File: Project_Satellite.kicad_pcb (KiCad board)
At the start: 4 copper layers, 40.2 x 65.5 mm, 83 parts, among them J1 Conn_01x02_Socket, J10 Conn_01x01_Socket, J11 Conn_01x01_Socket, J12 Conn_01x01_Socket, J13 Conn_01x01_Socket, J14 Conn_01x01_Socket, J15 Conn_01x01_Socket, J16 Conn_01x01_Socket, J17 Conn_01x01_Socket, J18 Conn_01x01_Socket, J19 Conn_01x01_Socket, J2 Conn_01x01_Socket, J20 Conn_01x01_Socket, J21 Conn_01x01_Socket, J22 Conn_01x01_Socket, J23 Conn_01x01_Socket, J24 Conn_01x01_Socket, J25 Conn_01x03_Socket, J26 Conn_01x03_Socket, J27 Conn_01x03_Socket, J28 Conn_01x03_Socket, J3 Conn_01x01_Socket, J4 Conn_01x01_Socket, J5 Conn_01x02_Socket, J6 Conn_01x02_Socket, J7 Conn_01x01_Socket, J8 Conn_01x02_Socket, J9 Conn_01x02_Socket, U3 TPS62933, U4 RASPBERRY_PI_ZERO_2_W, U5 TLV320AIC3254IRHBR, U6 MEMSMic, U7 MEMSMic, U8 TPA3118D2DAPR

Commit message: Final V1 commit
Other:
- copper layers 4 -> 2
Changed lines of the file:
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@@
 	(layers
 		(0 "F.Cu" signal)
-		(4 "In1.Cu" power "PWR.Cu")
-		(6 "In2.Cu" power "GND.Cu")
 		(2 "B.Cu" signal)
 		(9 "F.Adhes" user "F.Adhesive")
@@
 			)
 			(layer "dielectric 1"
-				(type "prepreg")
-				(thickness 0.1)
-				(material "FR4")
-				(epsilon_r 4.5)
-				(loss_tangent 0.02)
-			)
-			(layer "In1.Cu"
-				(type "copper")
-				(thickness 0.035)
-			)
-			(layer "dielectric 2"
 				(type "core")
-				(thickness 1.24)
-				(material "FR4")
-				(epsilon_r 4.5)
-				(loss_tangent 0.02)
-			)
-			(layer "In2.Cu"
-				(type "copper")
-				(thickness 0.035)
-			)
-			(layer "dielectric 3"
-				(type "prepreg")
-				(thickness 0.1)
+				(thickness 1.51)
 				(material "FR4")
 				(epsilon_r 4.5)
@@
 			(plot_on_all_layers_selection 0x00000000_00000000_00000000_00000000)
 			(disableapertmacros no)
-			(usegerberextensions no)
+			(usegerberextensions yes)
 			(usegerberattributes yes)
 			(usegerberadvancedattributes yes)
@@
 			(outputformat 1)
 			(mirror no)
-			(drillshape 1)
+			(drillshape 0)
 			(scaleselection 1)
-			(outputdirectory "")
+			(outputdirectory "V1_Fabrication/")
 		)
 	)

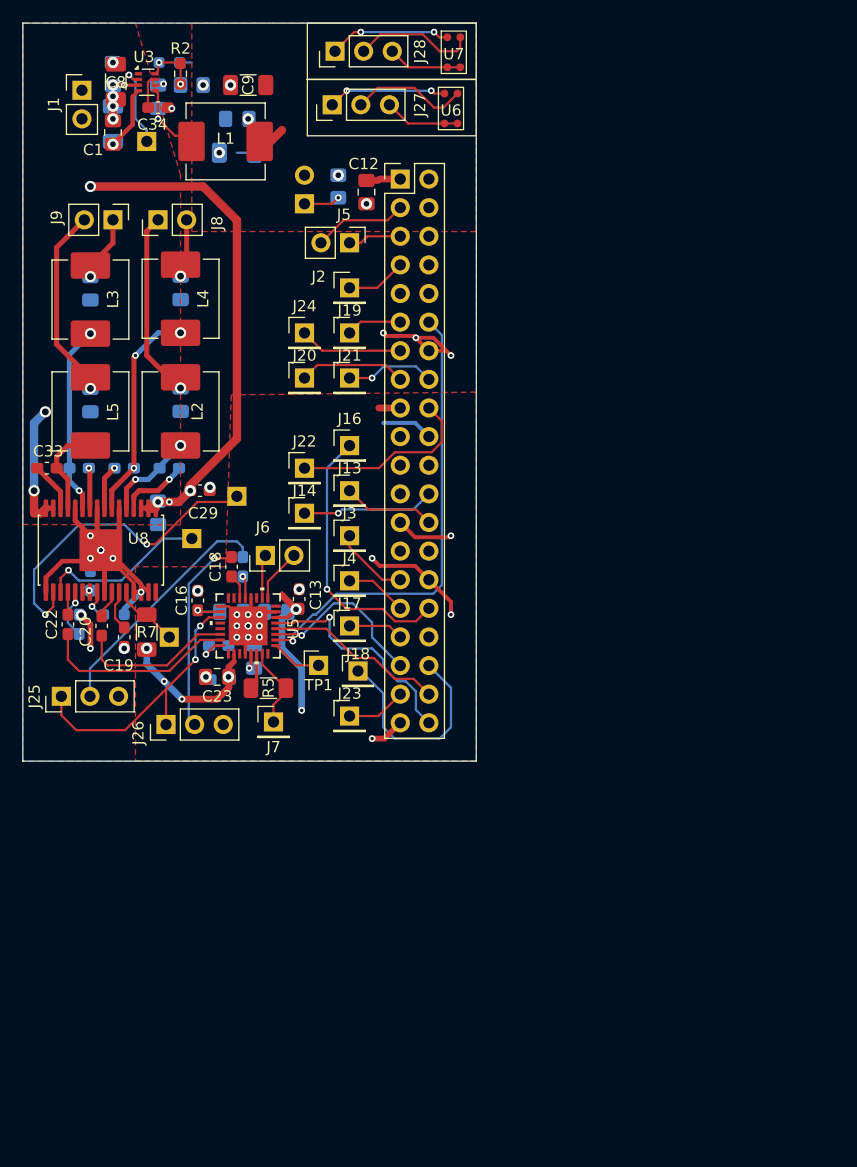
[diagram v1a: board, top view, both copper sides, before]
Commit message: TPA3118 changes
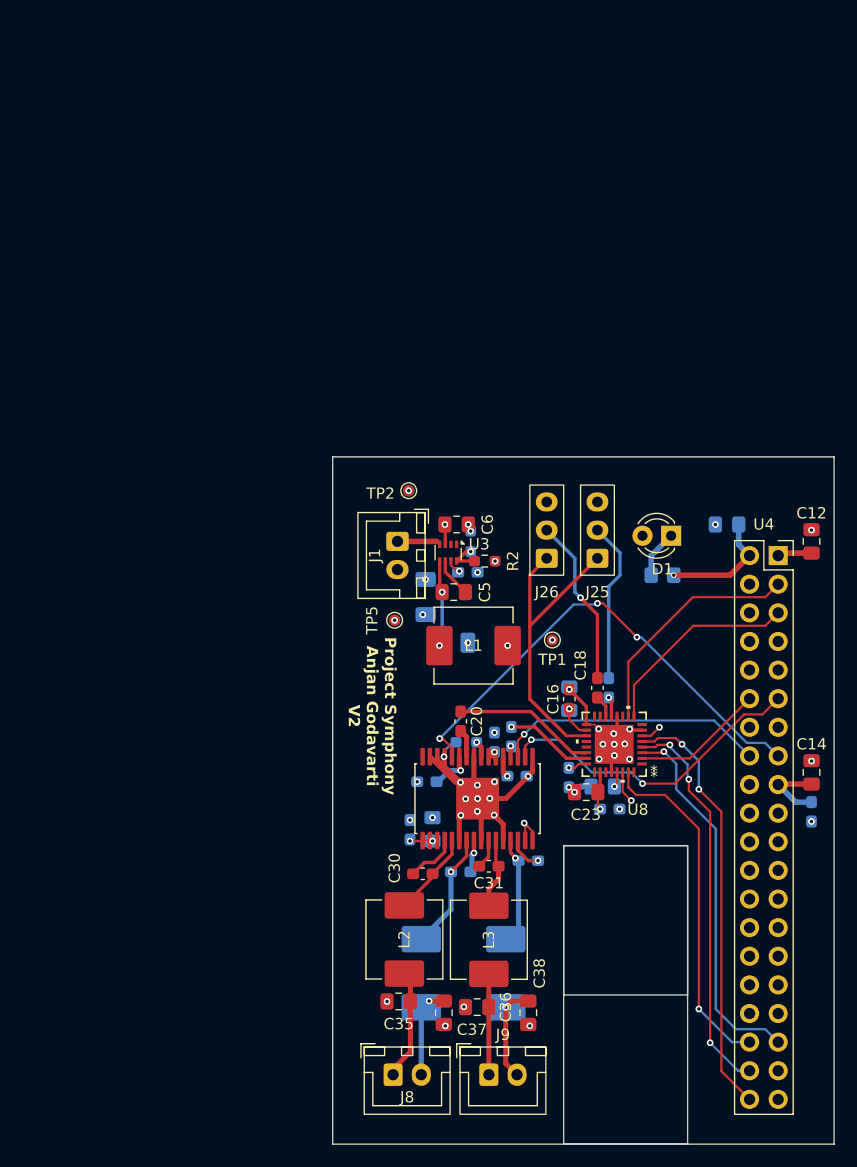
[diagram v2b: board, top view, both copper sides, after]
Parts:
- removed C11: 0.1uF, Capacitor_SMD:C_0805_2012Metric_Pad1.18x1.45mm_HandSolder
- removed C7: 10uF, Capacitor_SMD:C_1206_3216Metric_Pad1.33x1.80mm_HandSolder
- removed C9: 22uF, Capacitor_SMD:C_1206_3216Metric_Pad1.33x1.80mm_HandSolder
- removed J10, J11, J12, J13, J14, J15, J16, J17, J18, J19, J2, J20, J21, J22, J23, J24, J3, J4, J7: Conn_01x01_Socket, Connector_PinHeader_2.54mm:PinHeader_1x01_P2.54mm_Vertical
- removed J27, J28: Conn_01x03_Socket, Connector_PinHeader_2.54mm:PinHeader_1x03_P2.54mm_Vertical
- removed J5, J6: Conn_01x02_Socket, Connector_PinHeader_2.54mm:PinHeader_1x02_P2.54mm_Vertical
- removed R3: 50, Resistor_SMD:R_0805_2012Metric_Pad1.20x1.40mm_HandSolder
- removed R5, R7: 10k, Resistor_SMD:R_1206_3216Metric_Pad1.30x1.75mm_HandSolder
- removed U6, U7: MEMSMic, MyFootprints:MEMSMic
- added TP2: TestPoint, TestPoint:TestPoint_Pad_D1.0mm, F.Cu at (102.2, 64.0)
- added TP3: TestPoint, TestPoint:TestPoint_Pad_D1.0mm, B.Cu at (101.0, 75.5)
- added TP4: TestPoint, TestPoint:TestPoint_Pad_D1.0mm, B.Cu at (102.2, 64.0)
- added TP5: TestPoint, TestPoint:TestPoint_Pad_D1.0mm, F.Cu at (101.0, 75.5)
- C1, C13, C19, C22, C29, C33, C34, C8, L4, L5: moved to B.Cu
- C10: value 22uF -> 47uF
- C14, C30, C31, C35, C36, C37, C38, C5, C6: moved to F.Cu
- D1: footprint Connector_PinHeader_2.54mm:PinHeader_1x02_P2.54mm_Horizontal -> LED_THT:LED_D3.0mm; moved to F.Cu
- J1, J8, J9: footprint Connector_PinHeader_2.54mm:PinHeader_1x02_P2.54mm_Vertical -> Connector_JST:JST_XH_B2B-XH-A_1x02_P2.50mm_Vertical
- J25, J26: footprint Connector_PinHeader_2.54mm:PinHeader_1x03_P2.54mm_Vertical -> Connector_JST:JST_XH_B3B-XH-A_1x03_P2.50mm_Vertical
- TP1: footprint Connector_PinHeader_2.54mm:PinHeader_1x01_P2.54mm_Horizontal -> TestPoint:TestPoint_Pad_D1.0mm
- U4: footprint Connector_PinHeader_2.54mm:PinHeader_2x20_P2.54mm_Vertical -> Connector_PinSocket_2.54mm:PinSocket_2x20_P2.54mm_Vertical
- moved J9 82.9 mm to (109.4, 115.8), turned to 0 degrees
- moved J8 78.7 mm to (100.9, 115.8), turned to 0 degrees
- moved C36 72.4 mm to (108.3, 109.8), turned to 0 degrees
- moved C37 68.4 mm to (105.4, 110.3)
- moved L3 66.9 mm to (109.4, 103.9), turned to -90 degrees
- moved C38 66.8 mm to (112.9, 110.3)
- moved C1 64.7 mm to (130.5, 67.0), turned to 180 degrees
- moved L4 63.6 mm to (103.4, 106.8), turned to -90 degrees
- moved L5 62.0 mm to (110.9, 106.8), turned to -90 degrees
- moved C35 56.8 mm to (101.4, 109.3), turned to 0 degrees
- moved C33 55.1 mm to (112.9, 96.8), turned to 180 degrees
- moved C8 53.4 mm to (103.8, 73.4), turned to -90 degrees
- moved C5 51.2 mm to (106.2, 73.0), turned to 180 degrees
- moved R2 51.0 mm to (109.0, 70.2), turned to 0 degrees
- moved L2 50.9 mm to (101.9, 103.8), turned to -90 degrees
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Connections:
- C1 pad 1: +15V -> +5V
- C12 pad 2: +3V3 -> +3.3V
- R2 pad 2: Net-(U3-FB) -> +5V
- TP1 pad 1: Net-(U5-MCLK) -> +5V
- U3 pad 2: Net-(J15-Pin_1) -> unconnected-(U3-EN-Pad2)
- U4 pad 1: +3V3 -> +3.3V
- U4 pad 11: Net-(J19-Pin_1) -> /SDZ
- U4 pad 13: Net-(J24-Pin_1) -> unconnected-(U4-GPIO27/GPIO_GEN2-Pad13)
- U4 pad 15: Net-(J20-Pin_1) -> /MUTE
- U4 pad 16: Net-(J21-Pin_1) -> /FAULTZ
- U4 pad 18: Net-(J22-Pin_1) -> unconnected-(U4-GPIO24/GPIO_GEN5-Pad18)
- U4 pad 24: Net-(J14-Pin_1) -> unconnected-(U4-GPIO8/SPI_~{CE0}-Pad24)
- U4 pad 26: Net-(J13-Pin_1) -> unconnected-(U4-GPIO7/SPI_~{CE1}-Pad26)
- U4 pad 29: Net-(J3-Pin_1) -> unconnected-(U4-GPIO5-Pad29)
- U4 pad 3: Net-(J5-Pin_2) -> /SDA
- U4 pad 31: Net-(J4-Pin_1) -> unconnected-(U4-GPIO6-Pad31)
- U4 pad 32: Net-(J16-Pin_1) -> unconnected-(U4-GPIO12-Pad32)
- U4 pad 33: Net-(J17-Pin_1) -> unconnected-(U4-GPIO13-Pad33)
- U4 pad 36: Net-(J18-Pin_1) -> /RESET
- U4 pad 37: Net-(J23-Pin_1) -> unconnected-(U4-GPIO26-Pad37)
- U4 pad 5: Net-(J5-Pin_1) -> /SCL
- U4 pad 7: Net-(J2-Pin_1) -> unconnected-(U4-GPIO4/GPIO_GCLK-Pad7)
- U5 pad 1: Net-(U5-MCLK) -> unconnected-(U5-MCLK-Pad1)
- U5 pad 10: Net-(J6-Pin_1) -> /SDA
- U5 pad 31: Net-(J7-Pin_1) -> /RESET
- U5 pad 9: Net-(J6-Pin_2) -> /SCL
- U8 pad 12: Net-(J12-Pin_1) -> /MUTE
- U8 pad 2: Net-(J10-Pin_1) -> /SDZ
- U8 pad 3: Net-(J11-Pin_1) -> /FAULTZ
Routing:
- net +15V: track 62.1 -> 7.96 mm, vias 11 -> 6
- net GND: track 91.9 -> 45.8 mm, vias 38 -> 42
- net /MUTE: track 0.00 -> 42.8 mm, vias 0 -> 3
- net /RESET: track 0.00 -> 30.8 mm, vias 0 -> 1
- net Net-(U4-GPIO18/GPIO_GEN1): track 41.0 -> 11.8 mm, vias 1 -> 0
- net Net-(J10-Pin_1): track 28.8 -> 0.00 mm, vias 2 -> 0
- net /SDZ: track 0.00 -> 28.4 mm, vias 0 -> 2
- net Net-(J16-Pin_1): track 24.3 -> 0.00 mm, vias 1 -> 0
- net /FAULTZ: track 0.00 -> 24.0 mm, vias 0 -> 1
- net /SDA: track 0.00 -> 21.0 mm
- net Net-(U4-GPIO20): track 16.0 -> 35.3 mm, vias 0 -> 3
- net Net-(J18-Pin_1): track 18.9 -> 0.00 mm
- net Net-(U4-GPIO19): track 15.3 -> 33.6 mm
- net /SCL: track 0.00 -> 18.2 mm
- net Net-(U4-GPIO21): track 20.0 -> 37.9 mm, vias 1 -> 2
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- added copper zone on In1.Cu, net +15V
- added copper zone on In1.Cu, net +3.3V
- added copper zone on In1.Cu, net +5V
- added copper zone on In2.Cu, net GND
- removed copper zone on F.Cu, net +15V
- removed copper zone on F.Cu, net +3.3V
- removed copper zone on F.Cu, net +5V
- removed copper zone on B.Cu, net GND
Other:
- board size 40.2 x 65.5 mm -> 44.5 x 61 mm
- copper layers 2 -> 4
- board text added: "Project Symphony Anjan Godavarti V2"
- board text removed: "Project Symphony Anjan Godavarti V1"
